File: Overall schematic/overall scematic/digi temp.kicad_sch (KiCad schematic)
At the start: 5 parts

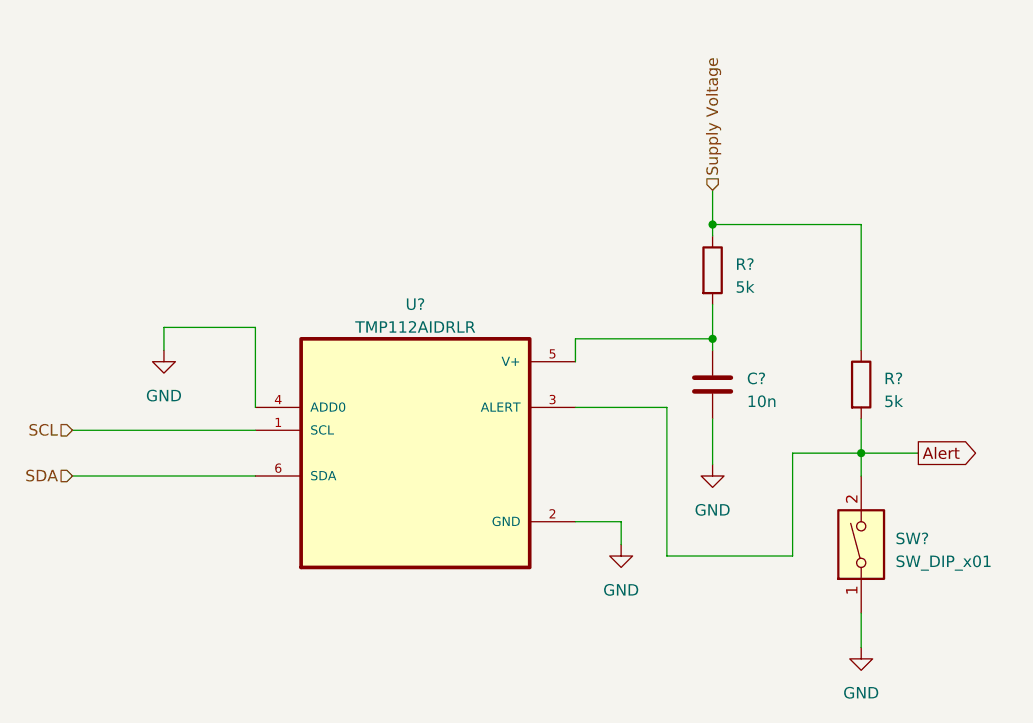
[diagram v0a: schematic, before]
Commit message: Add files via upload
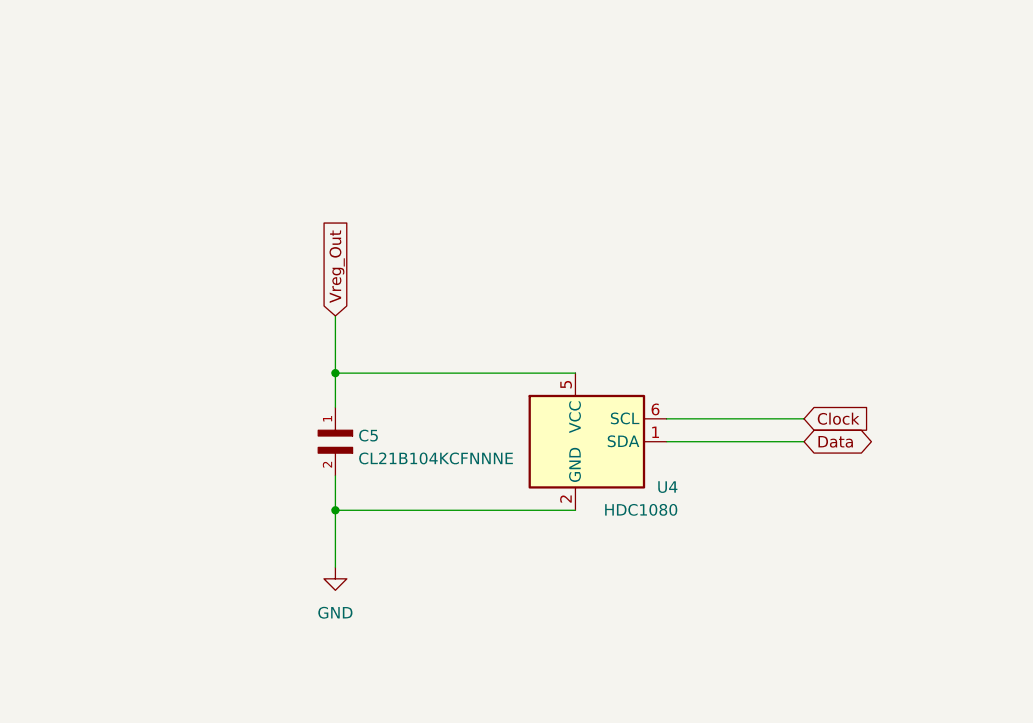
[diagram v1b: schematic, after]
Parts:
- removed C?: 10n, symbol Device:C
- removed R? (x2): 5k, symbol Device:R
- removed SW?: SW_DIP_x01, symbol Switch:SW_DIP_x01
- removed U?: TMP112AIDRLR, SOT50P160X60-6N, symbol TMP112AIDRLR:TMP112AIDRLR
- added C5: CL21B104KCFNNNE, CAPC2012X140N, symbol CL21B104KCFNNNE:CL21B104KCFNNNE
- added U4: HDC1080, Package_SON:Texas_PWSON-N6, symbol Sensor_Humidity:HDC1080
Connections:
- net GND: now also C5.2, U4.2 (GND)
- new net Clock: U4.6 (SCL)
- new net Data: U4.1 (SDA)
- new net Vreg_Out: C5.1, U4.5 (VCC)
